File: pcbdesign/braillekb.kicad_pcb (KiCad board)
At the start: 2 copper layers, 175.3 x 38.1 mm, 17 parts, among them SW11 SW_Push, SW12 SW_Push, SW23 SW_Push, SW24 SW_Push, SW47 SW_Push, SW48 SW_Push, SW55 SW_Push, SW56 SW_Push, U11 ProMicro

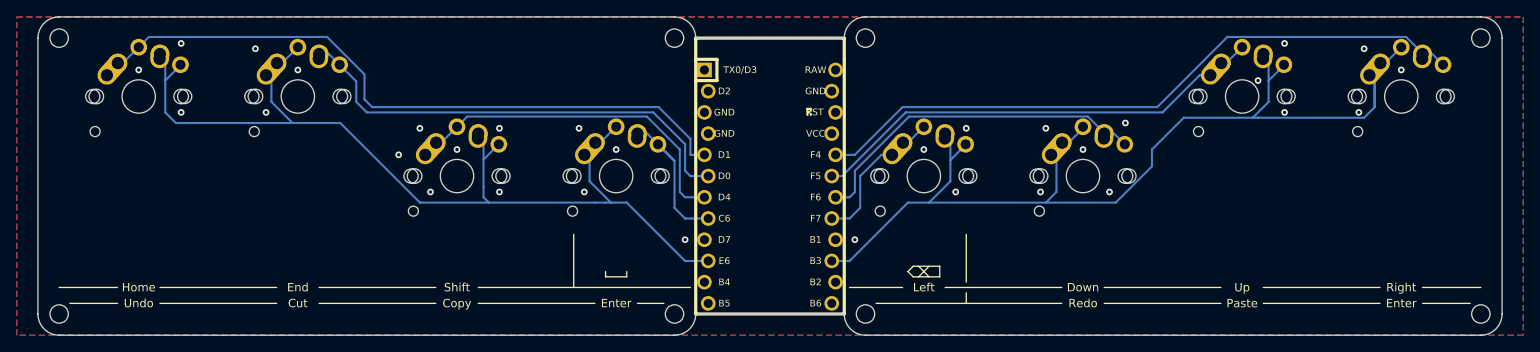
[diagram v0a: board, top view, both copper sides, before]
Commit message: modify route
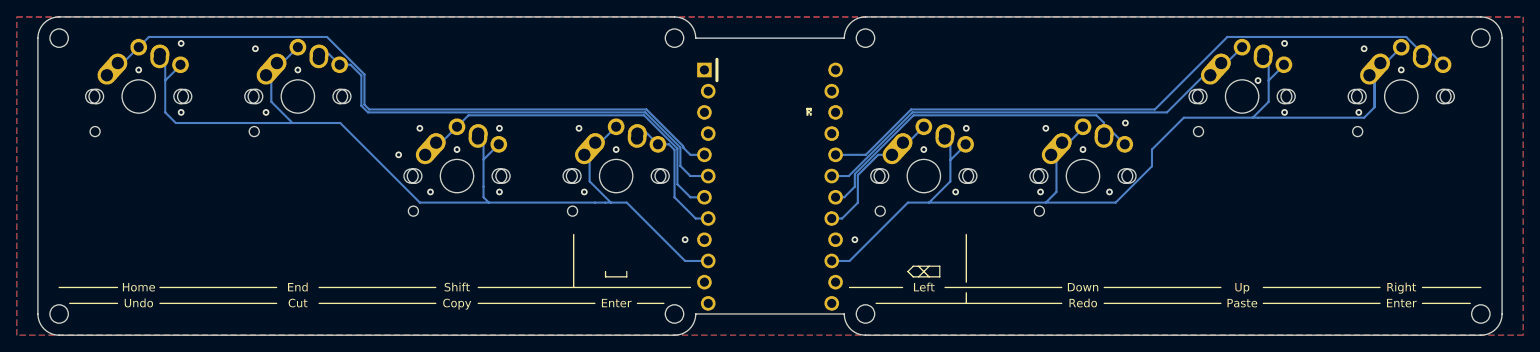
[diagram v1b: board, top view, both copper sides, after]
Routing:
- net C4: track 18.7 -> 16.0 mm
- net C6: track 41.4 -> 43.0 mm
- net C1: track 81.7 -> 81.0 mm
